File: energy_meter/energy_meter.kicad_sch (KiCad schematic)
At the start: 149 parts, among them IC1 ADUM4151BRIZ, IC2 ADUM6404ARIZ, IC3 ADP122AUJZ-3.3-R7, IC4 24LC32A_SN, J1 Screw_Terminal_01x02, J10 IB_in, J2 Screw_Terminal_01x02, J3 MicroUSB, J8 5V_SMPS, J9 IA_in, Q1 Q_NMOS_SGD, SW1 SW_Push, SW2 SW_Push, T1 IA_in, T2 IB_in, U1 ADE9000ACPZ, U2 SN74LV4T125PWR, U3 SN74LV4T125PWR, U4 Pico_SMD_NODEBUG, U5 BME280, U6 AMS1117-3.3, Y1 Crystal_GND24

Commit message: Restore libraries
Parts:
- U1: footprint ade9000:ADE9000ACPZ_ADI-M -> ADE9000:ADE9000ACPZ_ADI
- U2, U3: footprint SN74LV4T125PWR:PW0014A_N -> SN74LV:PW0014A_N
- U4: footprint RPi Pico:RPi_PicoW_SMD -> RPi_Pico:RPi_PicoW_SMD
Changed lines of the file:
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@@
       (effects (font (size 1.27 1.27)))
     )
-    (property "Footprint" "RPi Pico:RPi_PicoW_SMD" (at 224.79 320.04 90)
+    (property "Footprint" "RPi_Pico:RPi_PicoW_SMD" (at 224.79 320.04 90)
       (effects (font (size 1.27 1.27)) hide)
     )
@@
       (effects (font (size 1.524 1.524)))
     )
-    (property "Footprint" "SN74LV4T125PWR:PW0014A_N" (at 351.79 248.92 0)
+    (property "Footprint" "SN74LV:PW0014A_N" (at 351.79 248.92 0)
       (effects (font (size 1.27 1.27) italic) hide)
     )
@@
       (effects (font (size 1.524 1.524)))
     )
-    (property "Footprint" "SN74LV4T125PWR:PW0014A_N" (at 529.59 248.92 0)
+    (property "Footprint" "SN74LV:PW0014A_N" (at 529.59 248.92 0)
       (effects (font (size 1.27 1.27) italic) hide)
     )
@@
       (effects (font (size 1.524 1.524)))
     )
-    (property "Footprint" "ade9000:ADE9000ACPZ_ADI-M" (at 241.3 68.58 0)
+    (property "Footprint" "ADE9000:ADE9000ACPZ_ADI" (at 241.3 68.58 0)
       (effects (font (size 1.27 1.27) italic) hide)
     )

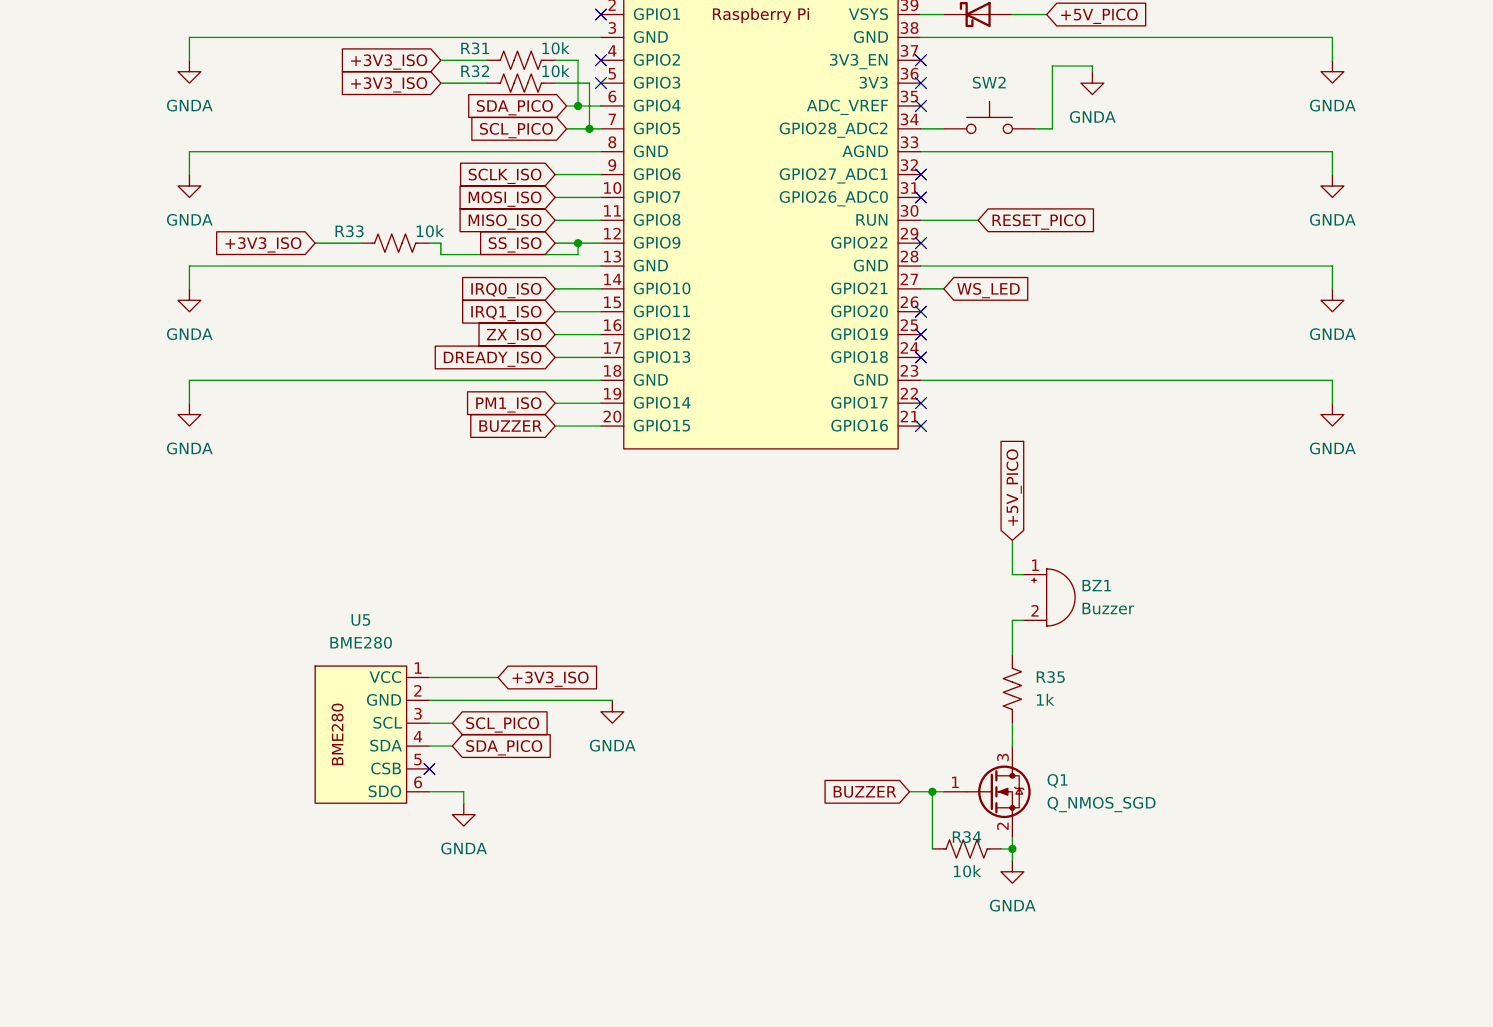
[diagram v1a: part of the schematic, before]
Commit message: more libraries
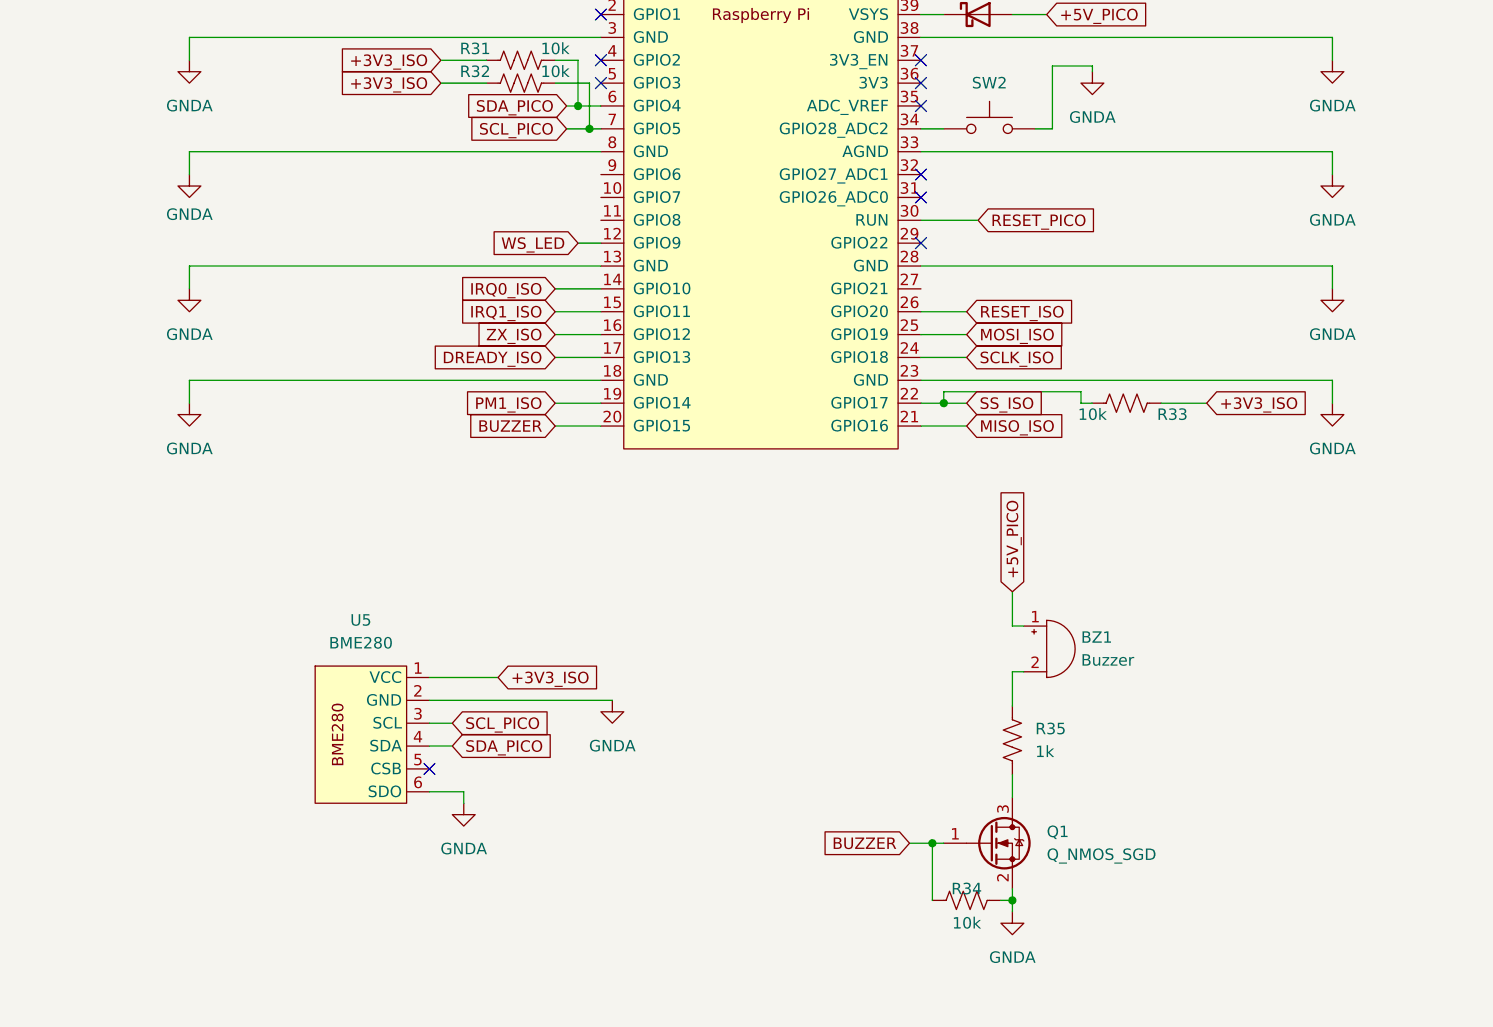
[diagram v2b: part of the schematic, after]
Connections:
- net MISO_ISO: now also U4.21 (GPIO16); no longer U4.11 (GPIO8)
- net MOSI_ISO: now also U4.25 (GPIO19); no longer U4.10 (GPIO7)
- net RESET_ISO: now also U4.26 (GPIO20)
- net SCLK_ISO: now also U4.24 (GPIO18); no longer U4.9 (GPIO6)
- net SS_ISO: now also U4.22 (GPIO17); no longer U4.12 (GPIO9)
- net WS_LED: now also U4.12 (GPIO9); no longer U4.27 (GPIO21)
- no-connect marks 32 -> 27
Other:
- moved on the sheet: BZ1, Q1, R34, R35
